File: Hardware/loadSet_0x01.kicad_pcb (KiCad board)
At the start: 2 copper layers, 88.3 x 76.2 mm, 45 parts, among them J1 Conn_01x05, J2 Conn_01x01, J3 Conn_01x01, J4 Conn_01x01, J5 Conn_01x01, Q1 Q_NMOS_GDS, Q2 Q_NMOS_GDS, U1 OPA2333xxDGK, U2 OPA2333xxDGK

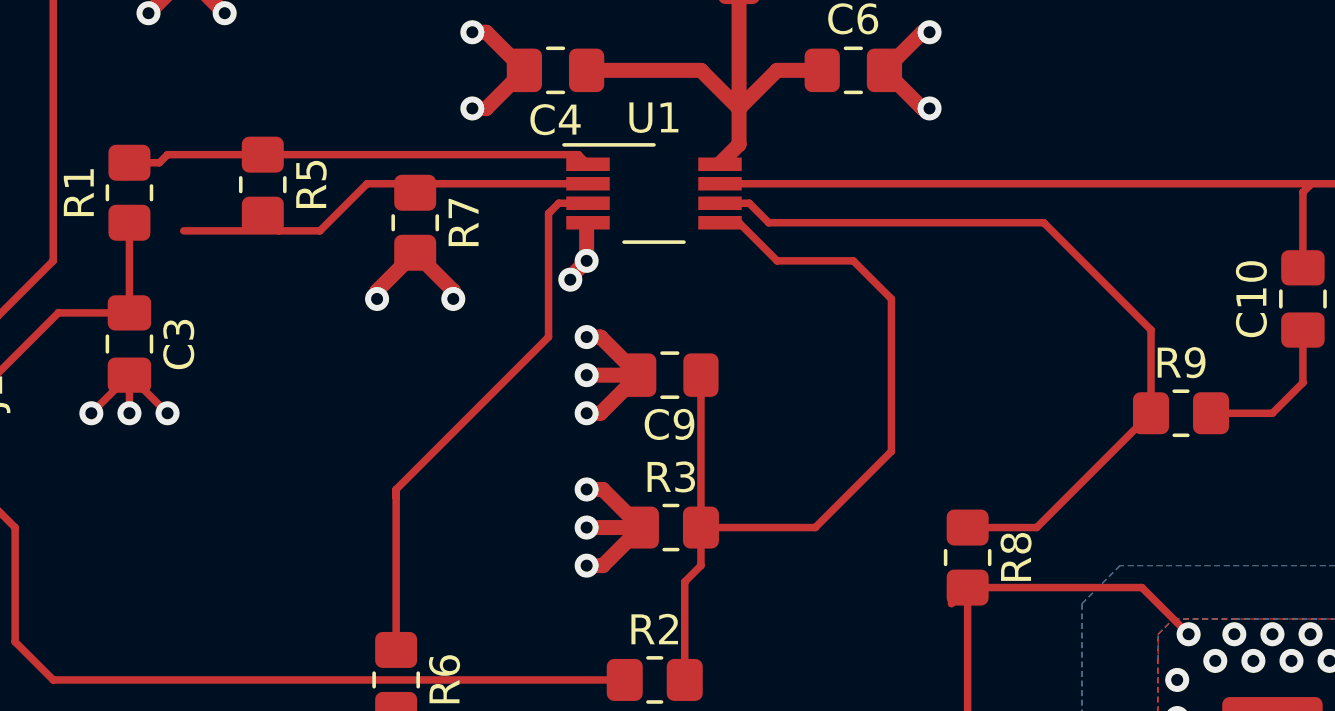
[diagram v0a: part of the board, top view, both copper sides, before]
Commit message: additional code and values
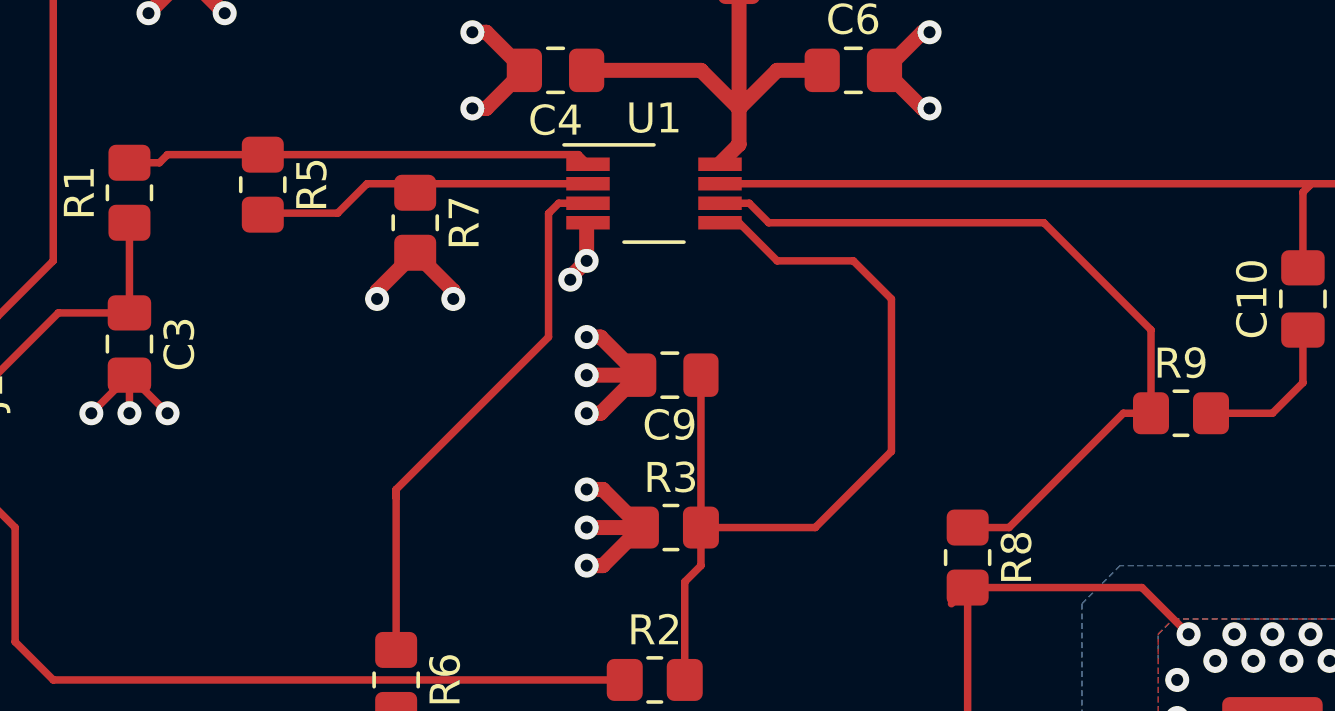
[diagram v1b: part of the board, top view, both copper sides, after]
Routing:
- net Net-(R5-Pad2): track 15.2 -> 11.6 mm
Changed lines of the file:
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@@
   (segment (start 85.755 71.12) (end 86.065 71.43) (width 0.25) (layer "F.Cu") (net 13))
   (segment (start 86.065 70.78) (end 86.065 70.81) (width 0.25) (layer "F.Cu") (net 13))
-  (segment (start 81.185 84.09) (end 80.645 83.55) (width 0.25) (layer "F.Cu") (net 14))
+  (segment (start 80.695 83.5) (end 80.645 83.55) (width 0.25) (layer "F.Cu") (net 14))
   (segment (start 85.725 82.55) (end 85.755 82.52) (width 0.25) (layer "F.Cu") (net 14))
+  (segment (start 83.14 83.5) (end 80.695 83.5) (width 0.25) (layer "F.Cu") (net 14))
   (segment (start 85.725 82.82) (end 85.725 82.55) (width 0.25) (layer "F.Cu") (net 14))
   (segment (start 85.755 82.52) (end 84.12 82.52) (width 0.25) (layer "F.Cu") (net 14))
   (segment (start 91.485 82.52) (end 85.755 82.52) (width 0.25) (layer "F.Cu") (net 14))
-  (segment (start 84.12 82.52) (end 82.55 84.09) (width 0.25) (layer "F.Cu") (net 14))
-  (segment (start 82.55 84.09) (end 78.01 84.09) (width 0.25) (layer "F.Cu") (net 14))
+  (segment (start 84.12 82.52) (end 83.14 83.5) (width 0.25) (layer "F.Cu") (net 14))
   (segment (start 90.17 83.51) (end 90.17 87.63) (width 0.25) (layer "F.Cu") (net 15))
   (segment (start 90.17 87.63) (end 85.09 92.71) (width 0.25) (layer "F.Cu") (net 15))
@@
   (segment (start 90.51 83.17) (end 90.17 83.51) (width 0.25) (layer "F.Cu") (net 15))
   (segment (start 95.885 83.17) (end 96.86 83.17) (width 0.25) (layer "F.Cu") (net 16))
-  (segment (start 106.442 93.98) (end 110.252 90.17) (width 0.25) (layer "F.Cu") (net 16))
+  (segment (start 105.52 93.98) (end 109.33 90.17) (width 0.25) (layer "F.Cu") (net 16))
   (segment (start 97.51 83.82) (end 106.68 83.82) (width 0.25) (layer "F.Cu") (net 16))
   (segment (start 96.86 83.17) (end 97.51 83.82) (width 0.25) (layer "F.Cu") (net 16))
   (segment (start 110.252 87.392) (end 110.252 90.17) (width 0.25) (layer "F.Cu") (net 16))
+  (segment (start 104.14 93.98) (end 105.52 93.98) (width 0.25) (layer "F.Cu") (net 16))
   (segment (start 106.68 83.82) (end 110.252 87.392) (width 0.25) (layer "F.Cu") (net 16))
-  (segment (start 104.14 93.98) (end 106.442 93.98) (width 0.25) (layer "F.Cu") (net 16))
+  (segment (start 109.33 90.17) (end 110.252 90.17) (width 0.25) (layer "F.Cu") (net 16))
   (segment (start 101.6 70.12) (end 102.6 70.12) (width 0.25) (layer "F.Cu") (net 17))
   (segment (start 87.63 73.66) (end 88.9 74.93) (width 0.25) (layer "F.Cu") (net 17))
@@
     (connect_pads (clearance 0.508))
     (min_thickness 0.254) (filled_areas_thickness no)
-    (fill yes (thermal_gap 0.508) (thermal_bridge_width 0.508))
+    (fill yes (thermal_gap 0.108) (thermal_bridge_width 0.508))
     (polygon
       (pts
